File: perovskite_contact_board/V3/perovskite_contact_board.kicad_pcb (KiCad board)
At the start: 2 copper layers, 55.2 x 55.2 mm, 31 parts, among them U1 Perovskite_CP_6_Cell, U2 Perovskite_CP_6_Cell, U3 Perovskite_CP_6_Cell, U4 MCP9808_MSOP, U5 MCP9808_MSOP, U6 MCP9808_MSOP

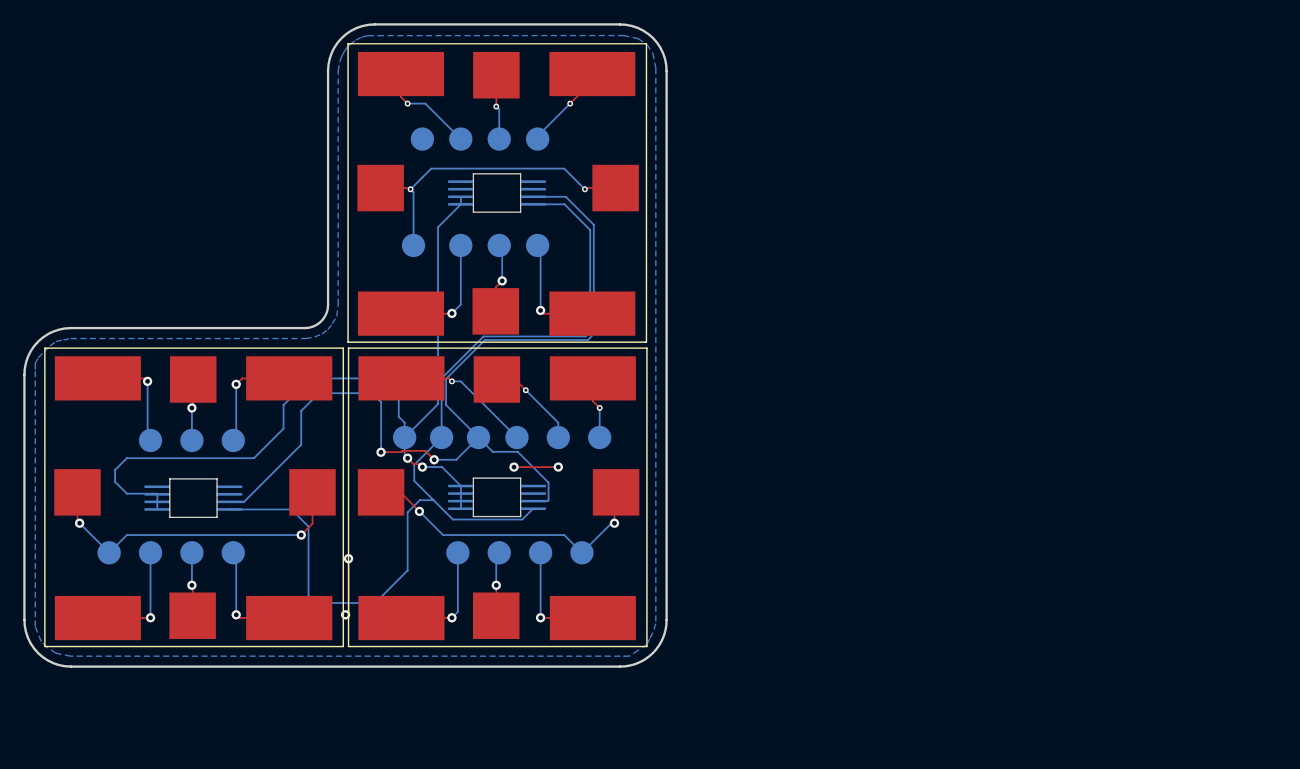
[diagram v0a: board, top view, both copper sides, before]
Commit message: Review contact board
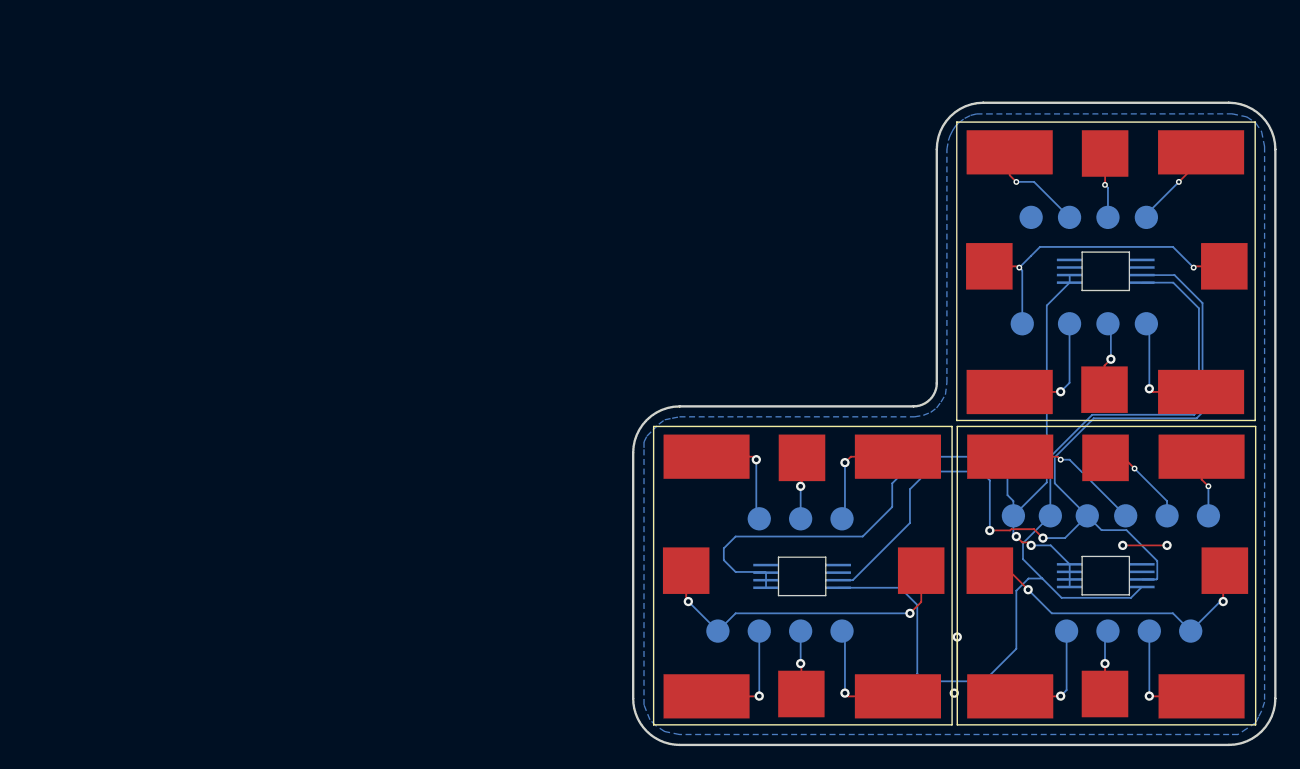
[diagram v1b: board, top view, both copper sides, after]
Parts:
- moved JP100.7 52.8 mm to (159.3, 98.7)
- moved JP101.3 52.8 mm to (143.8, 115.4)
- moved JP101.4 52.8 mm to (143.8, 125.1)
- moved JP102.2 52.8 mm to (171.7, 115.2)
- moved JP102.4 52.8 mm to (170.2, 125.1)
- moved JP102.6 52.8 mm to (163.1, 125.1)
- moved JP103.1 52.8 mm to (160.0, 89.5)
- moved JP103.2 52.8 mm to (158.5, 115.2)
- moved U4 52.8 mm to (166.4, 94.2)
- moved U5 52.8 mm to (140.3, 120.4)
- moved U6 52.8 mm to (166.4, 120.3)
- moved JP100.1 52.8 mm to (163.3, 89.5)
- moved JP100.2 52.8 mm to (166.6, 89.5)
- moved JP100.5 52.8 mm to (166.6, 98.7)
- moved JP100.6 52.8 mm to (163.3, 98.7)
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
